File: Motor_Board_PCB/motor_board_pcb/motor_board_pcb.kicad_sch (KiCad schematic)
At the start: 13 parts, among them U1 MCP2515-xST, U2 TJA1050, Y1 20M

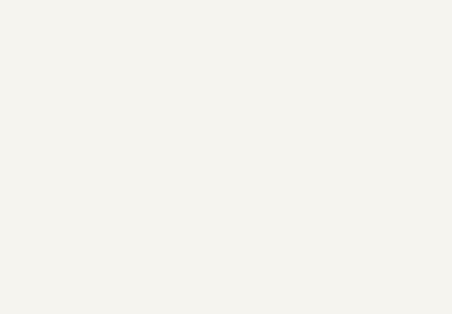
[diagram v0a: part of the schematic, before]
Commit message: added balls
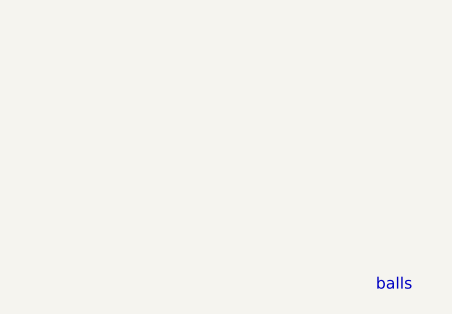
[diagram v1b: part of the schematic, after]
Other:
- note added: "balls"
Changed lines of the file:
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@@
+    (effects (font (size 1.27 1.27)) (justify left bottom))
+  )
+  (text "balls" (at 184.15 176.53 0)
     (effects (font (size 1.27 1.27)) (justify left bottom))
   )
